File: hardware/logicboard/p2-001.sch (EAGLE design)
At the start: 35 parts, among them IC1 5V, IC2 4066N, IC3 LTC485N, IC4 74LS07N, K1 G5V1, T1 2SC1815, U1 DS18B20

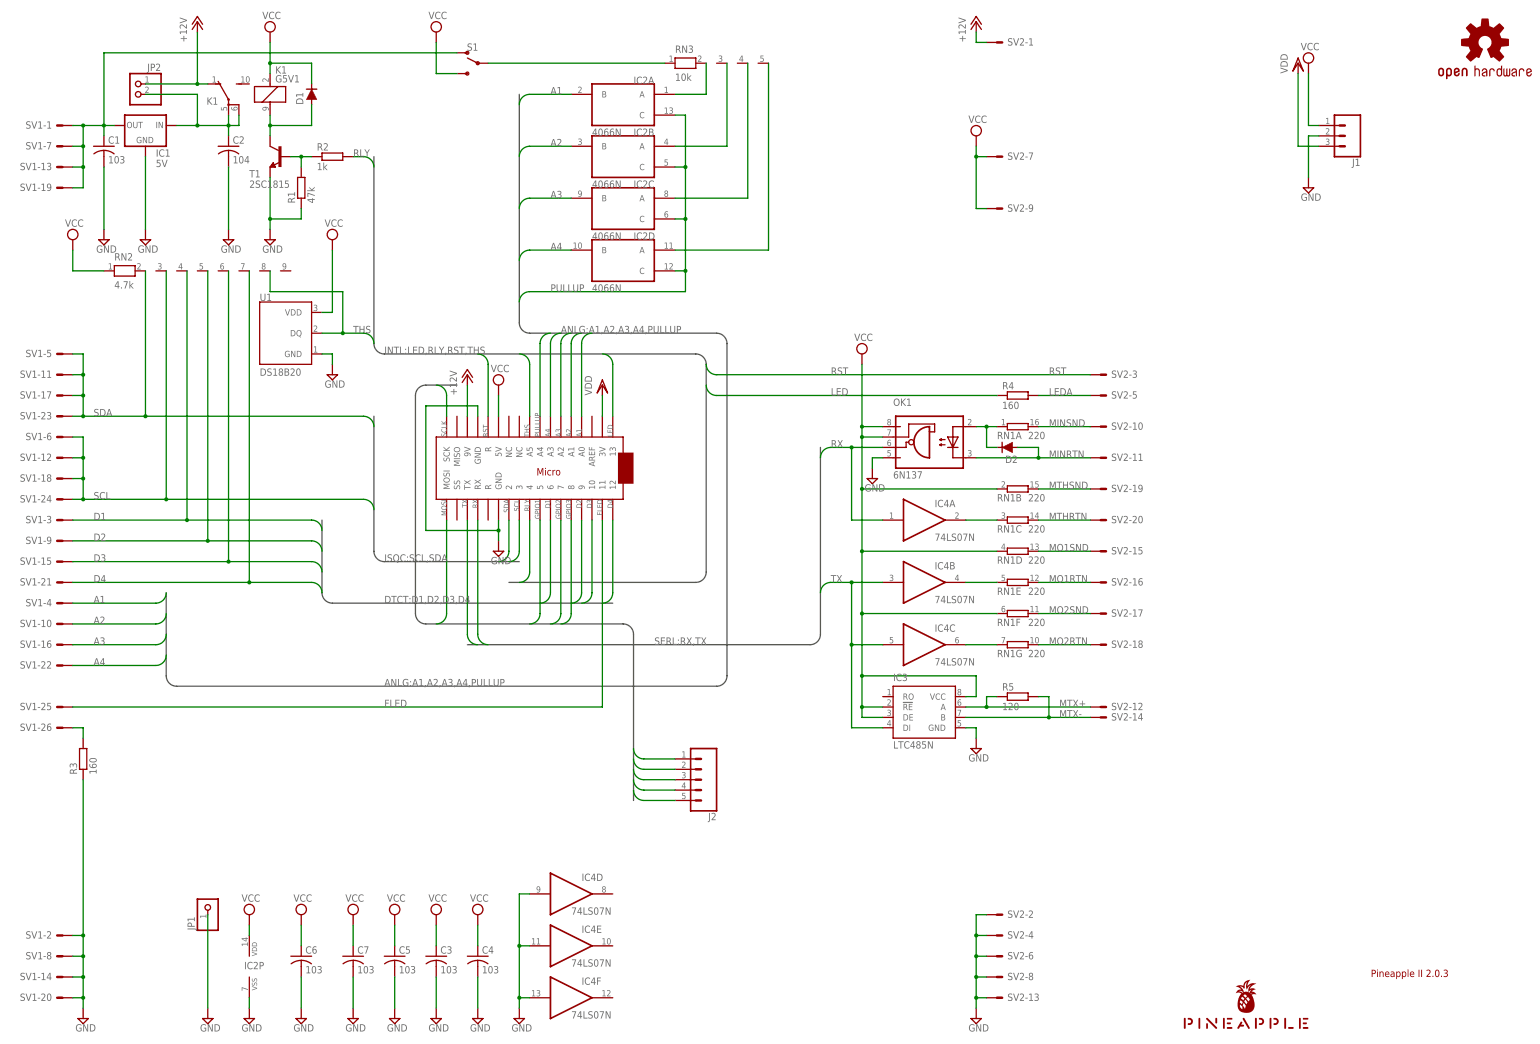
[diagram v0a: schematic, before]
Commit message: Readability.
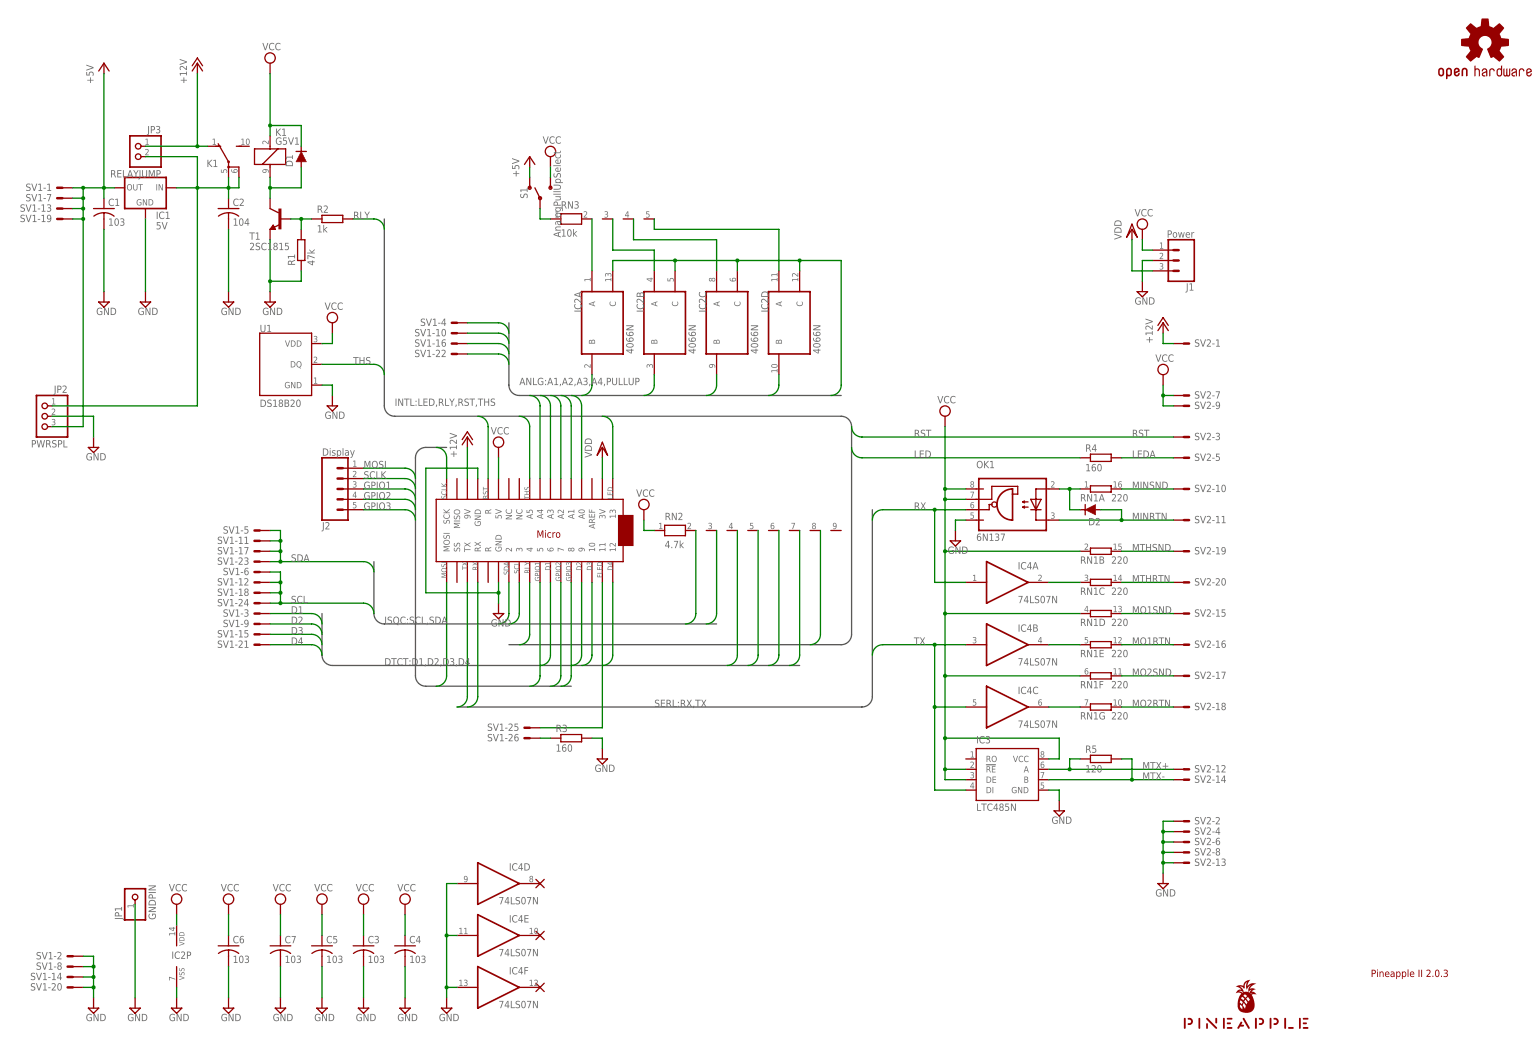
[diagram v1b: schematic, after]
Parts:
- added JP3: RELAYJUMP, pinhead:PINHD-1X2
- J1: value (none) -> Power
- J2: value (none) -> Display
- JP1: value (none) -> GNDPIN
- JP2: value (none) -> PWRSPL; device pinhead:PINHD-1X2 -> pinhead:PINHD-1X3
- S1: value (none) -> AnalogPullUpSelect
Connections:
- removed net FLEDK: R3.2, SV1-26.S
- removed net V+12V: C2.1, IC1.IN, JP2.2, K12.P, K12.P@1
- removed net VOUT: C1.1, IC1.OUT, S1.O, SV1-1.S, SV1-13.S, SV1-19.S, SV1-7.S
- new net +5V: C1.1, IC1.OUT, JP2.3, S1.O, SV1-1.S, SV1-13.S, SV1-19.S, SV1-7.S
- new net N$2: R3.1, SV1-26.S
- new net VIN: C2.1, IC1.IN, JP2.1, JP3.2, K12.P, K12.P@1
- net +12V: now also JP3.1; no longer JP2.1
- net GND: now also JP2.2, R3.2; no longer R3.1
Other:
- moved on the sheet: C1, C2, C3, C4, C5, C6, C7, D1, D2, IC1, IC2A, IC2B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
